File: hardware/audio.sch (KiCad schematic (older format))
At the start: 22 parts, among them U4 FM8002A, U5 TM8211, U6 FM8002A

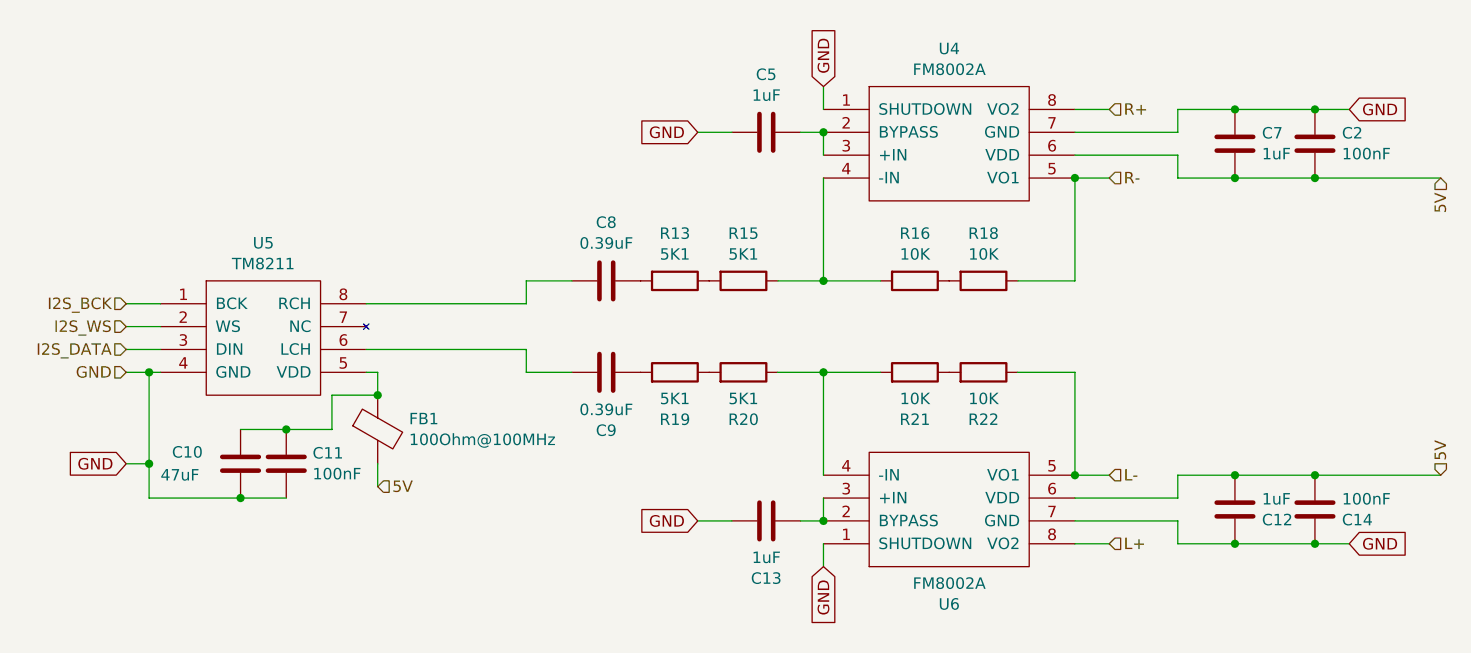
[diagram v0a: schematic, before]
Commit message: Wrover fp
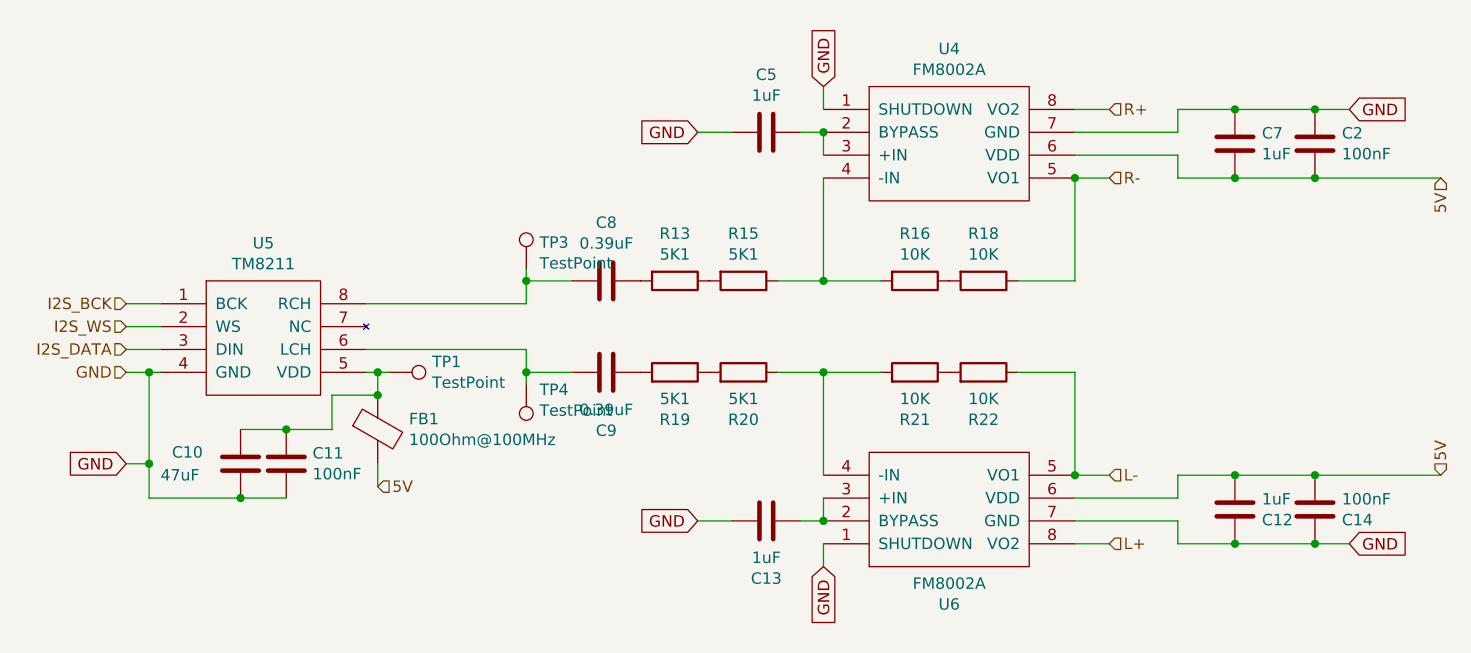
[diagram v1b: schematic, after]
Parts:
- added TP1, TP3, TP4: TestPoint, TestPoint:TestPoint_Pad_D1.5mm, symbol Connector:TestPoint
- C8, C9: LCSC (none) -> C1623
- FB1: footprint Inductor_SMD:L_0603_1608Metric -> Inductor_SMD:L_0805_2012Metric; LCSC (none) -> C1017
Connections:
- net at C10.1, C11.1, FB1.1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: now also TP1.1
- net at C9.2, U5.6 (LCH): now also TP4.1
- net at C8.2, U5.8 (RCH): now also TP3.1
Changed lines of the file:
@@
 F 2 "Capacitor_SMD:C_0603_1608Metric" H 3438 2900 50  0001 C CNN
 F 3 "~" H 3400 3050 50  0001 C CNN
+F 4 "C1623" H 3400 3050 50  0001 C CNN "LCSC"
 	1    3400 3050
 	0    1    1    0
@@
 F 2 "Capacitor_SMD:C_0603_1608Metric" H 3438 3300 50  0001 C CNN
 F 3 "~" H 3400 3450 50  0001 C CNN
+F 4 "C1623" H 3400 3450 50  0001 C CNN "LCSC"
 	1    3400 3450
 	0    1    -1   0
@@
 F 0 "FB1" H 2537 3746 50  0000 L CNN
 F 1 "100Ohm@100MHz" H 2537 3655 50  0000 L CNN
-F 2 "Inductor_SMD:L_0603_1608Metric" V 2330 3700 50  0001 C CNN
+F 2 "Inductor_SMD:L_0805_2012Metric" V 2330 3700 50  0001 C CNN
 F 3 "~" H 2400 3700 50  0001 C CNN
+F 4 "C1017" H 2400 3700 50  0001 C CNN "LCSC"
 	1    2400 3700
 	1    0    0    -1
@@
 Wire Wire Line
 	6500 2600 7050 2600
+$Comp
+L Connector:TestPoint TP1
+U 1 1 5E48F618
+P 2450 3450
+F 0 "TP1" V 2404 3638 50  0000 L CNN
+F 1 "TestPoint" V 2495 3638 50  0000 L CNN
+F 2 "TestPoint:TestPoint_Pad_D1.5mm" H 2650 3450 50  0001 C CNN
+F 3 "~" H 2650 3450 50  0001 C CNN
+	1    2450 3450
+	0    1    1    0
+$EndComp
+Wire Wire Line
+	2450 3450 2400 3450
+Connection ~ 2400 3450
+$Comp
+L Connector:TestPoint TP3
+U 1 1 5E4920BF
+P 3050 3000
+F 0 "TP3" H 3108 3118 50  0000 L CNN
+F 1 "TestPoint" H 3108 3027 50  0000 L CNN
+F 2 "TestPoint:TestPoint_Pad_D1.5mm" H 3250 3000 50  0001 C CNN
+F 3 "~" H 3250 3000 50  0001 C CNN
+	1    3050 3000
+	1    0    0    -1
+$EndComp
+Wire Wire Line
+	3050 3000 3050 3050
+Connection ~ 3050 3050
+$Comp
+L Connector:TestPoint TP4
+U 1 1 5E493FE0
+P 3050 3500
+F 0 "TP4" H 2992 3526 50  0000 R CNN
+F 1 "TestPoint" H 2992 3617 50  0000 R CNN
+F 2 "TestPoint:TestPoint_Pad_D1.5mm" H 3250 3500 50  0001 C CNN
+F 3 "~" H 3250 3500 50  0001 C CNN
+	1    3050 3500
+	-1   0    0    1
+$EndComp
+Wire Wire Line
+	3050 3500 3050 3450
+Connection ~ 3050 3450
 $EndSCHEMATC
